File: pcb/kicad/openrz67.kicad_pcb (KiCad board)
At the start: 2 copper layers, 48 x 22 mm, 59 parts, among them U1 ESP32-C3FH4, U3 LGS5500EP, U4 S4B-XH-A(LF)(SN), U5 TLP172GM, U6 TLP172GM, X1 40MHz, X2 32.768kHz

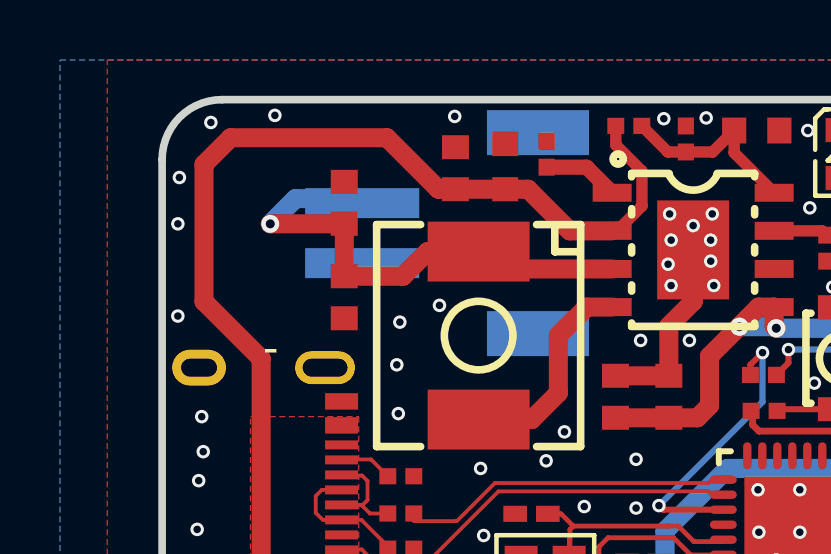
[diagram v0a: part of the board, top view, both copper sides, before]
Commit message: Update rev 2 PCB layout
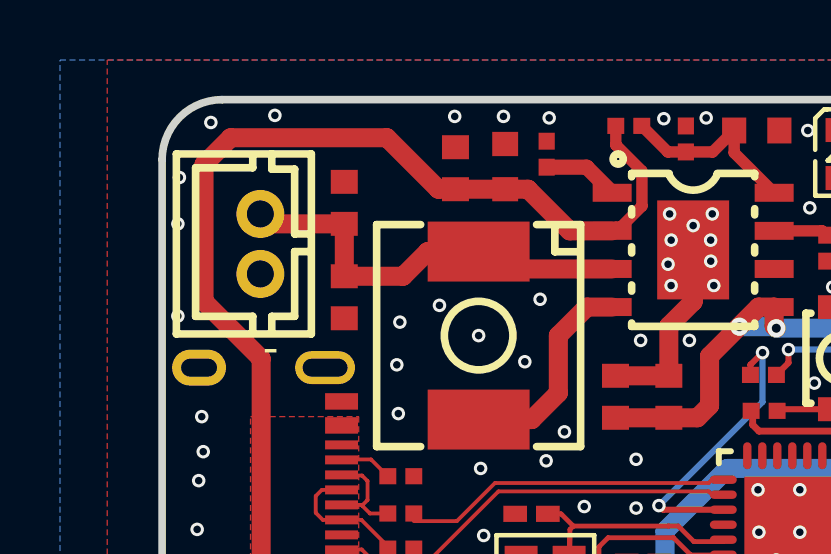
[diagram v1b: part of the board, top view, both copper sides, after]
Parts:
- BAT1: value S2B-PH-SM4-TB(LF)(SN) -> B2B-PH-K-S(LF)(SN); footprint openrz67:CONN-SMD_P2.00_S2B-PH-SM4-TB-LF-SN -> openrz67:CONN-TH_B2B-PH-K-S; moved to F.Cu
- moved BAT1 6.34 mm to (123.3, 94.8), turned to 90 degrees
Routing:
- net BAT+: track 17.1 -> 14.2 mm, vias 1 -> 0
- net GND: vias 103 -> 108
